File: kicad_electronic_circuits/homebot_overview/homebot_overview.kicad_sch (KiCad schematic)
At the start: 5 parts, among them J1 Raspberry_Pi_4, M1 Motor_Servo, U1 TB6612FNG, U2 BNO055, U3 PCA9635

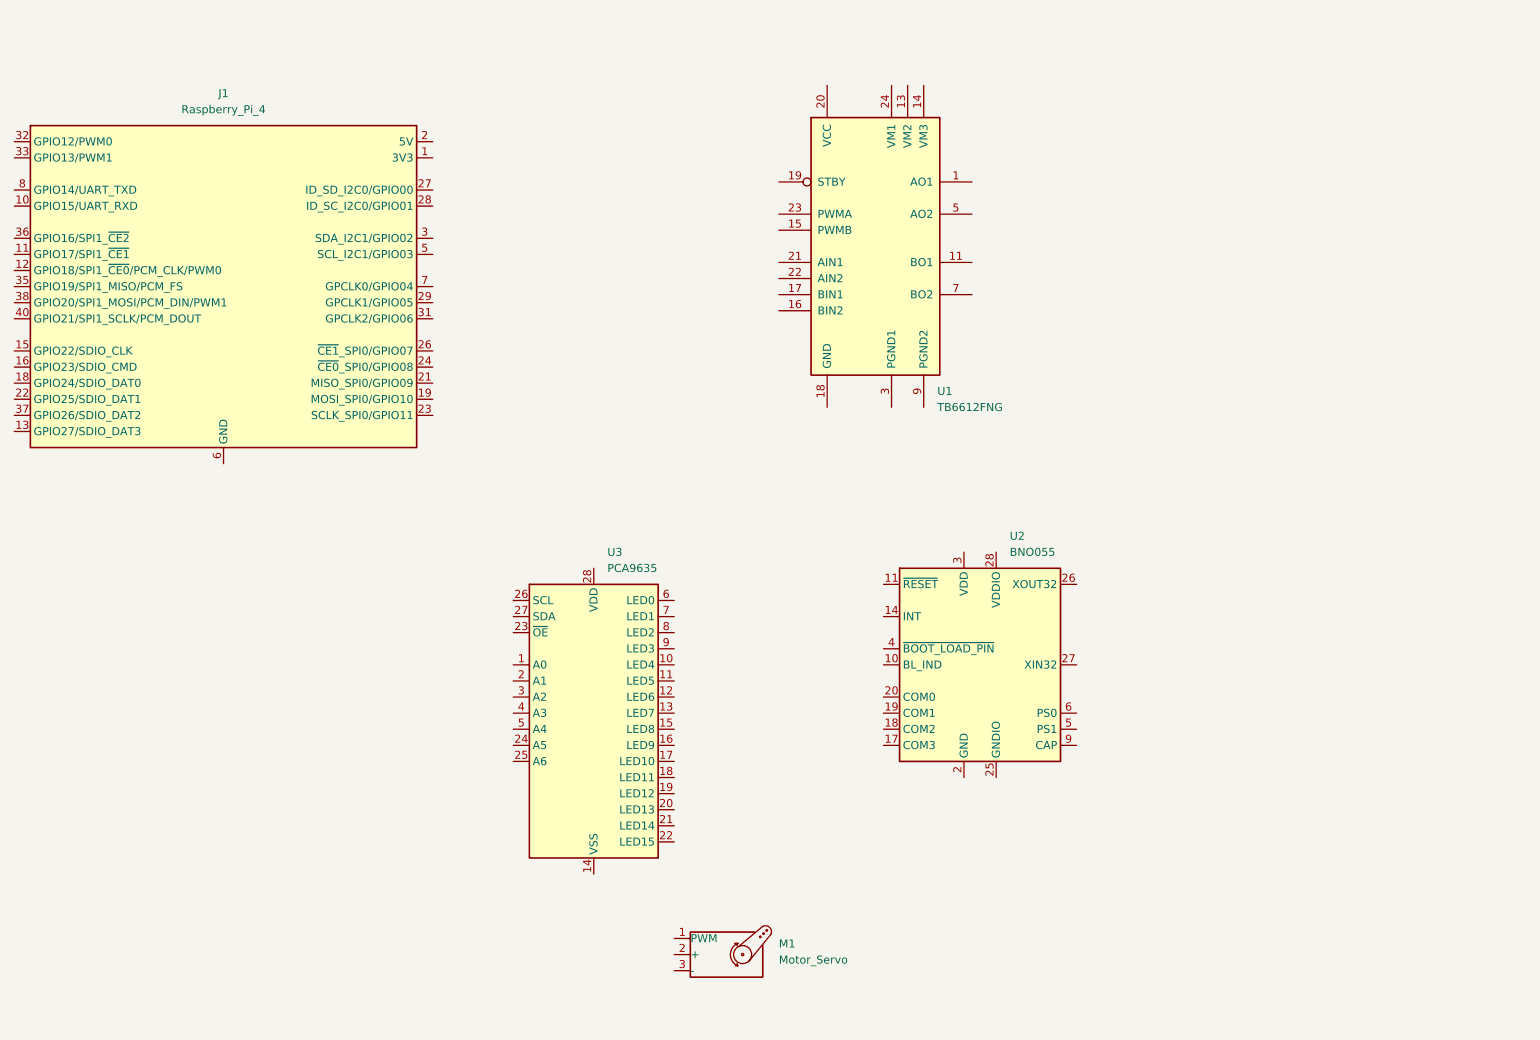
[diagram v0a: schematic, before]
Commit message: doc update
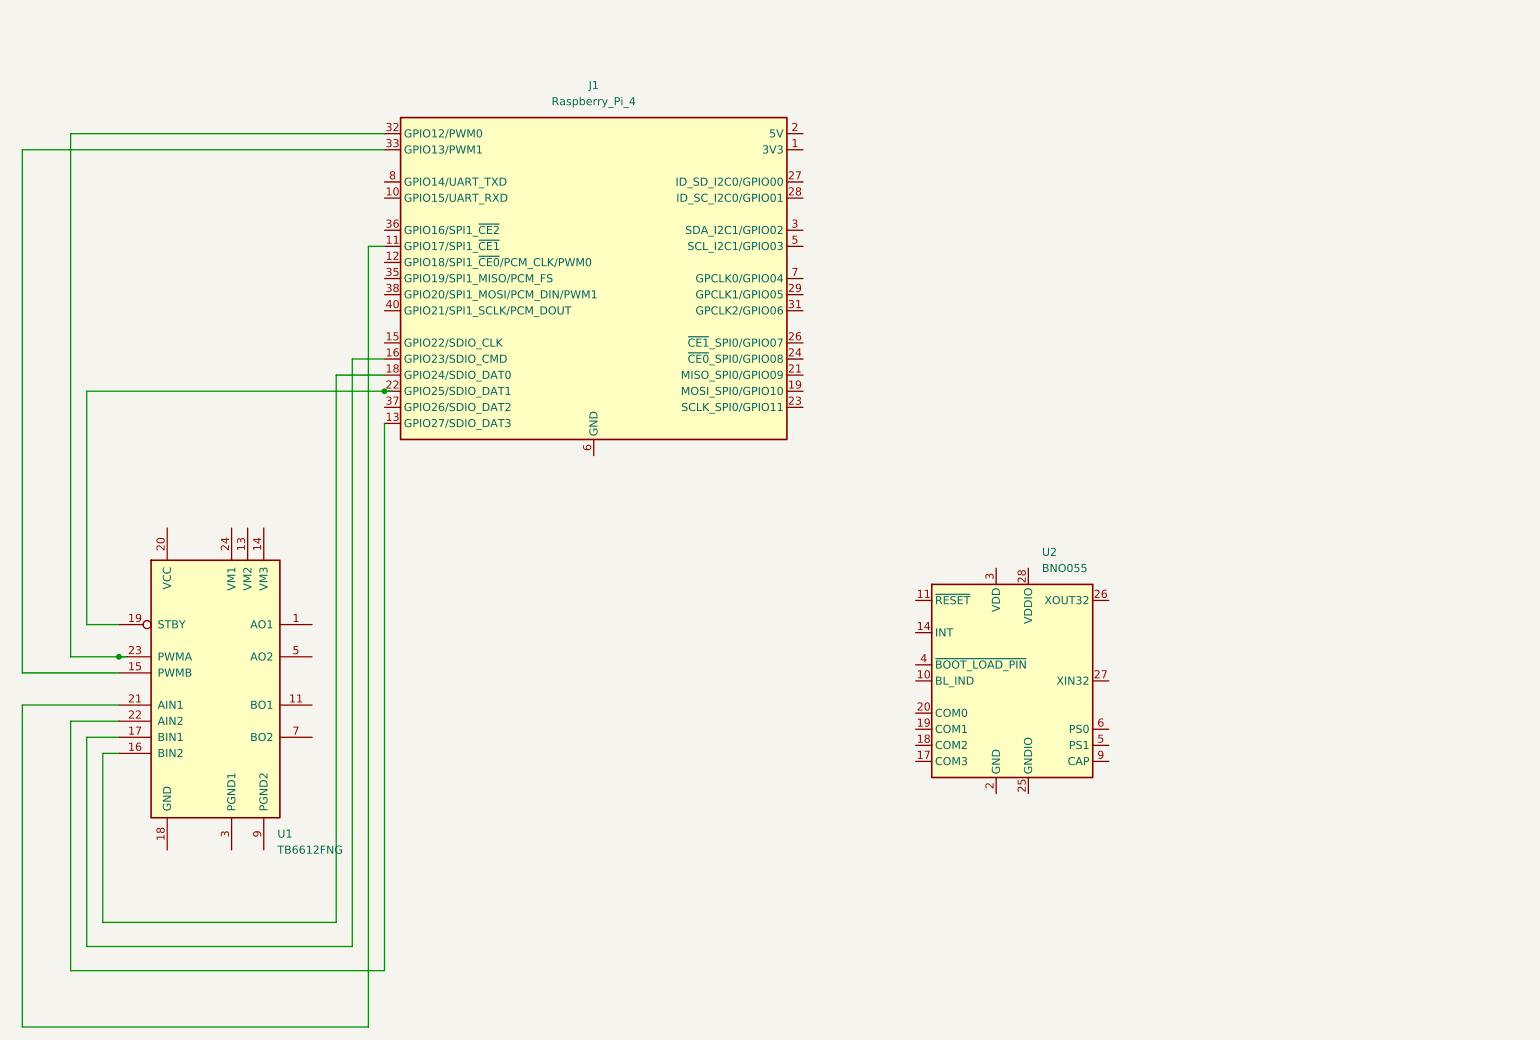
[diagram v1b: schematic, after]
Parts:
- removed M1: Motor_Servo, symbol Motor:Motor_Servo
- removed U3: PCA9635, Package_SO:TSSOP-28_4.4x9.7mm_P0.65mm, symbol Driver_LED:PCA9635
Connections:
- net at U1.15 (PWMB): now also J1.33 (GPIO13/PWM1)
- net at U1.16 (BIN2): now also J1.18 (GPIO24/SDIO_DAT0)
- net at U1.17 (BIN1): now also J1.16 (GPIO23/SDIO_CMD)
- net at U1.19 (STBY): now also J1.22 (GPIO25/SDIO_DAT1)
- net at U1.21 (AIN1): now also J1.11 (GPIO17/SPI1_~{CE1})
- net at U1.22 (AIN2): now also J1.13 (GPIO27/SDIO_DAT3)
- net at U1.23 (PWMA): now also J1.32 (GPIO12/PWM0)
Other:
- moved on the sheet: J1, U1, U2

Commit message: made some progress on overview schematic
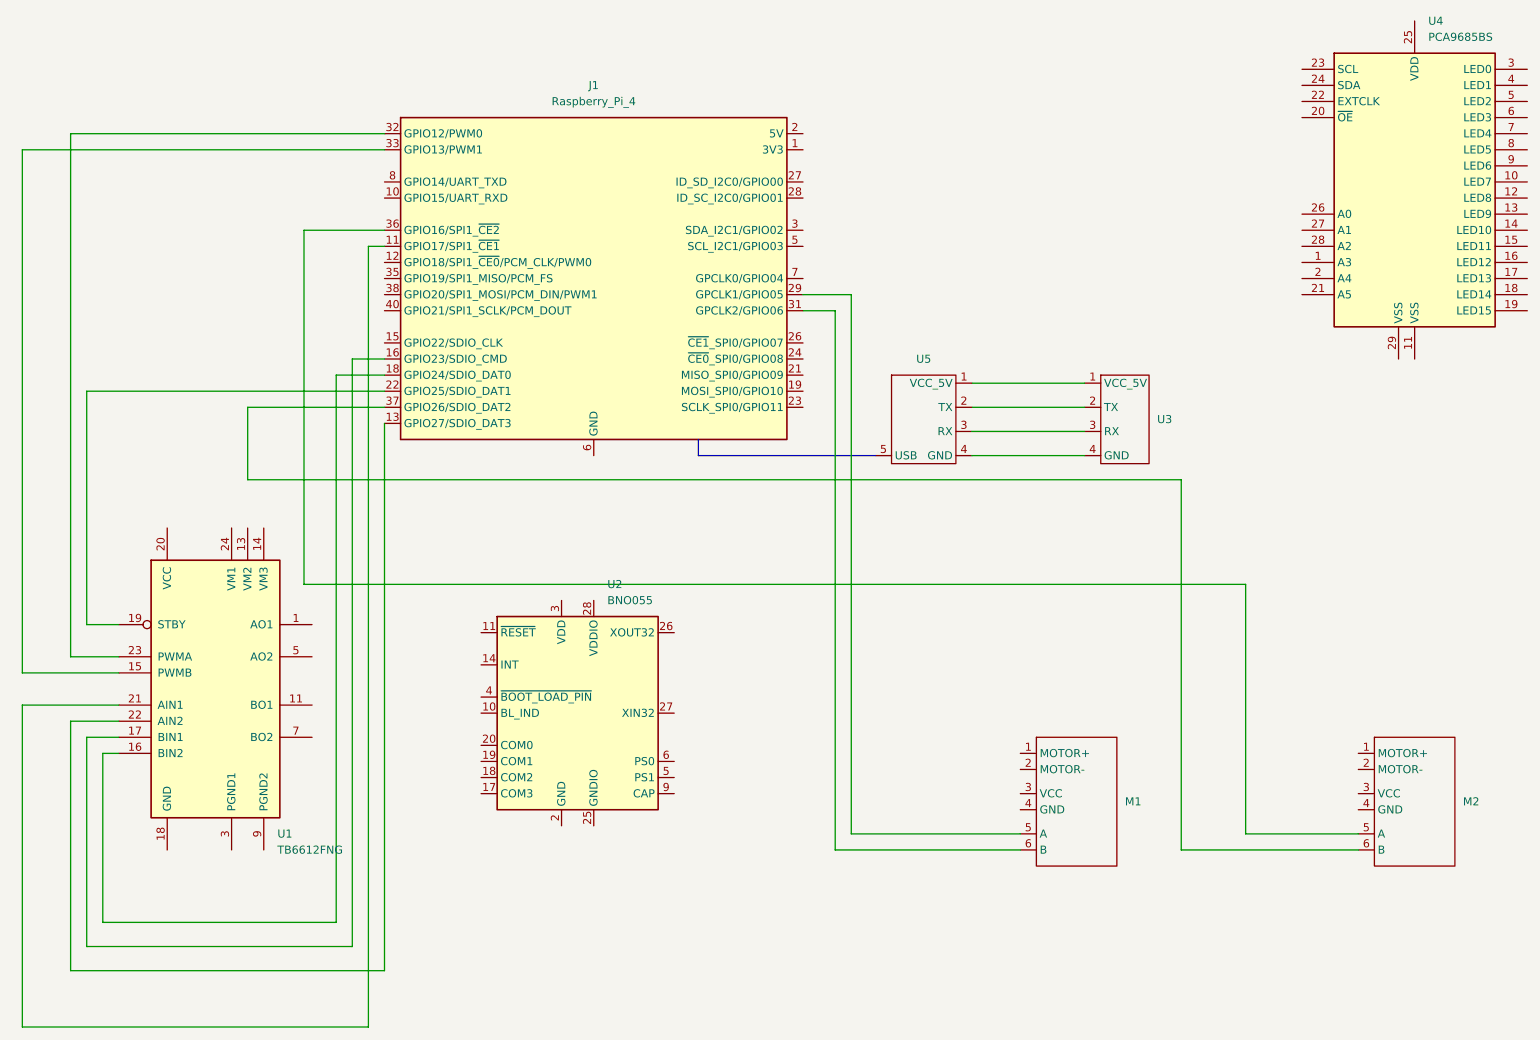
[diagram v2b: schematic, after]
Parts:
- added M1, M2: (no value), symbol homebot_symbols:TT_Motor_Encoder
- added U3: (no value), symbol homebot_symbols:RPLidarC1
- added U4: PCA9685BS, Package_DFN_QFN:QFN-28-1EP_6x6mm_P0.65mm_EP4.25x4.25mm, symbol Driver_LED:PCA9685BS
- added U5: (no value), symbol homebot_symbols:RPLIDAR_USB_ADAPTER
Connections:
- net at J1.29 (GPCLK1/GPIO05): now also M1.5 (A)
- net at J1.31 (GPCLK2/GPIO06): now also M1.6 (B)
- net at J1.36 (GPIO16/SPI1_~{CE2}): now also M2.5 (A)
- net at J1.37 (GPIO26/SDIO_DAT2): now also M2.6 (B)
- new net: U3.1 (VCC_5V), U5.1 (VCC_5V)
- new net: U3.2 (TX), U5.2 (TX)
- new net: U3.3 (RX), U5.3 (RX)
- new net: U3.4 (GND), U5.4 (GND)
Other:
- moved on the sheet: U2
